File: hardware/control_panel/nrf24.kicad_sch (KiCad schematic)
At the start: 6 parts, among them J11 Conn_02x04_Odd_Even, U10 SPX3819M5-L-3-3

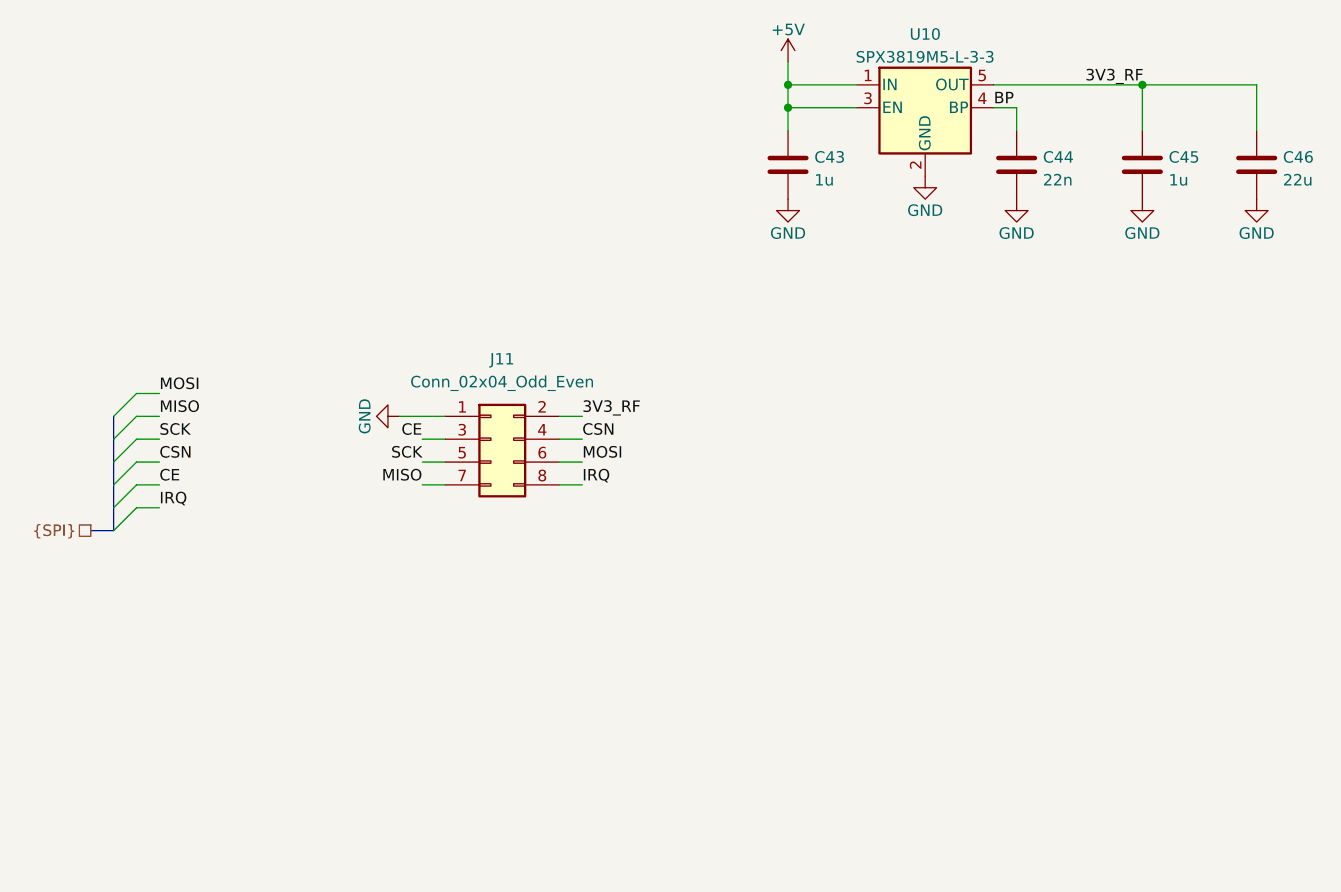
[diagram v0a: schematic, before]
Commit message: hw layout
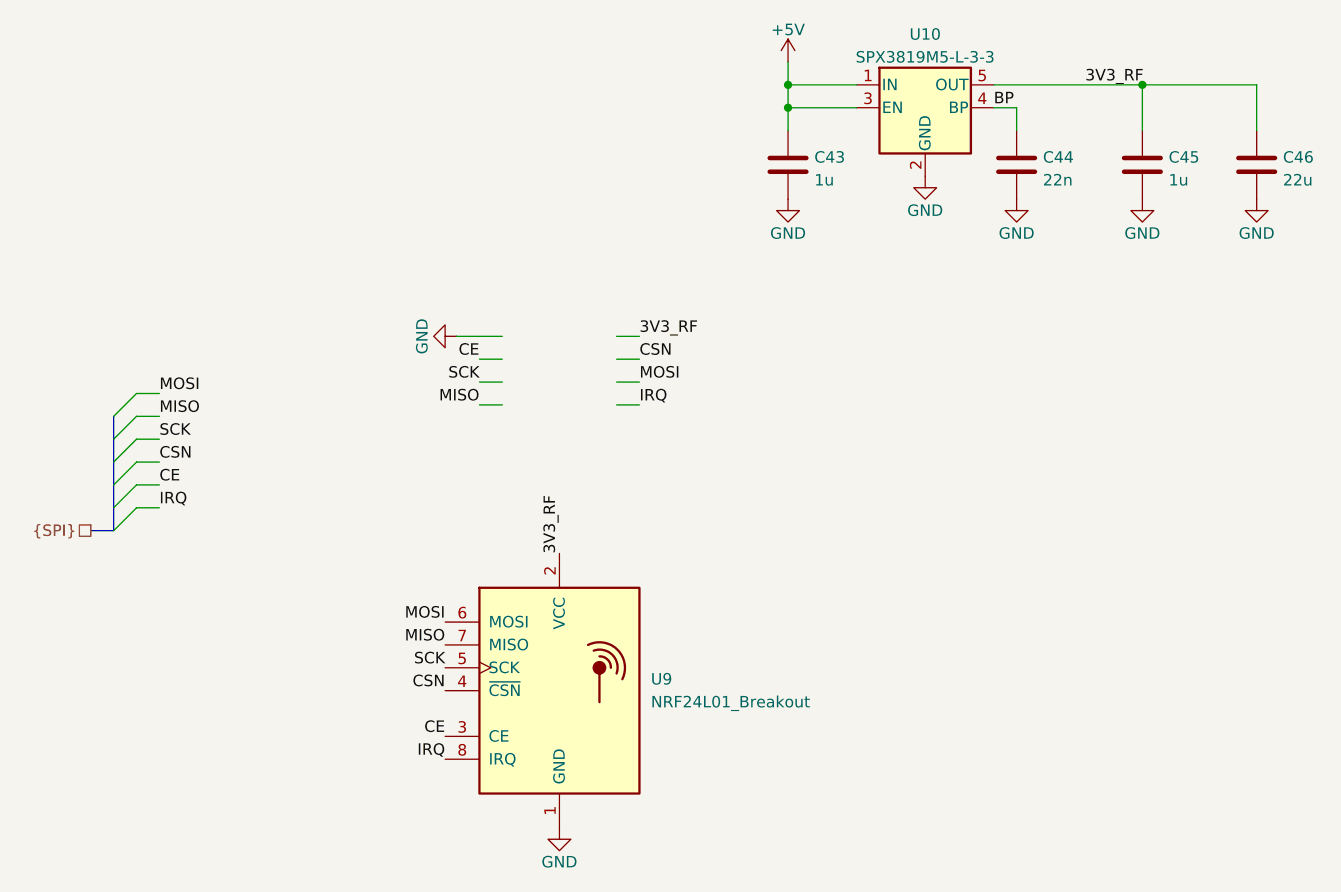
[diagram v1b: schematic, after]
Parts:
- removed J11: Conn_02x04_Odd_Even, Connector_PinSocket_2.54mm:PinSocket_2x04_P2.54mm_Vertical, symbol Connector_Generic:Conn_02x04_Odd_Even
- added U9: NRF24L01_Breakout, project_footprints:nRF24L01_Breakout, symbol RF:NRF24L01_Breakout
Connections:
- net 3V3_RF: now also U9.2 (VCC)
- net CE: now also U9.3 (CE)
- net CSN: now also U9.4 (~{CSN})
- net GND: now also U9.1 (GND)
- net IRQ: now also U9.8 (IRQ)
- net MISO: now also U9.7 (MISO)
- net MOSI: now also U9.6 (MOSI)
- net SCK: now also U9.5 (SCK)
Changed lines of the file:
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@@
     (stroke (width 0) (type default))
   )
-  (wire (pts (xy 113.03 81.28) (xy 110.49 81.28))
-    (stroke (width 0) (type default))
-  )
-  (wire (pts (xy 113.03 83.82) (xy 110.49 83.82))
-    (stroke (width 0) (type default))
-  )
-  (wire (pts (xy 95.25 81.28) (xy 97.79 81.28))
+  (wire (pts (xy 119.38 72.39) (xy 116.84 72.39))
+    (stroke (width 0) (type default))
+  )
+  (wire (pts (xy 119.38 74.93) (xy 116.84 74.93))
+    (stroke (width 0) (type default))
+  )
+  (wire (pts (xy 101.6 72.39) (xy 104.14 72.39))
     (stroke (width 0) (type default))
   )
@@
     (stroke (width 0) (type default))
   )
-  (wire (pts (xy 113.03 76.2) (xy 110.49 76.2))
+  (wire (pts (xy 119.38 67.31) (xy 116.84 67.31))
     (stroke (width 0) (type default))
   )
@@
     (stroke (width 0) (type default))
   )
-  (wire (pts (xy 113.03 78.74) (xy 110.49 78.74))
+  (wire (pts (xy 119.38 69.85) (xy 116.84 69.85))
     (stroke (width 0) (type default))
   )
@@
     (stroke (width 0) (type default))
   )
-  (wire (pts (xy 92.71 76.2) (xy 97.79 76.2))
-    (stroke (width 0) (type default))
-  )
-  (wire (pts (xy 95.25 78.74) (xy 97.79 78.74))
+  (wire (pts (xy 99.06 67.31) (xy 104.14 67.31))
+    (stroke (width 0) (type default))
+  )
+  (wire (pts (xy 101.6 69.85) (xy 104.14 69.85))
     (stroke (width 0) (type default))
   )
@@
     (stroke (width 0) (type default))
   )
-  (wire (pts (xy 95.25 83.82) (xy 97.79 83.82))
+  (wire (pts (xy 101.6 74.93) (xy 104.14 74.93))
     (stroke (width 0) (type default))
   )
@@
     (stroke (width 0) (type default))
   )
-  (label "MISO" (at 95.25 83.82 180) (fields_autoplaced)
+  (label "MISO" (at 101.6 74.93 180) (fields_autoplaced)
     (effects (font (size 1.27 1.27)) (justify right bottom))
   )
@@
     (effects (font (size 1.27 1.27)) (justify left bottom))
   )
-  (label "CSN" (at 113.03 78.74 0) (fields_autoplaced)
-    (effects (font (size 1.27 1.27)) (justify left bottom))
+  (label "IRQ" (at 97.79 114.3 180) (fields_autoplaced)
+    (effects (font (size 1.27 1.27)) (justify right bottom))
+  )
+  (label "CSN" (at 119.38 69.85 0) (fields_autoplaced)
+    (effects (font (size 1.27 1.27)) (justify left bottom))
+  )
+  (label "CSN" (at 97.79 106.68 180) (fields_autoplaced)
+    (effects (font (size 1.27 1.27)) (justify right bottom))
   )
   (label "CE" (at 66.04 83.82 0) (fields_autoplaced)
@@
     (effects (font (size 1.27 1.27)) (justify left bottom))
   )
-  (label "SCK" (at 95.25 81.28 180) (fields_autoplaced)
+  (label "SCK" (at 101.6 72.39 180) (fields_autoplaced)
     (effects (font (size 1.27 1.27)) (justify right bottom))
   )
@@
     (effects (font (size 1.27 1.27)) (justify left bottom))
   )
-  (label "3V3_RF" (at 113.03 76.2 0) (fields_autoplaced)
+  (label "MISO" (at 97.79 101.6 180) (fields_autoplaced)
+    (effects (font (size 1.27 1.27)) (justify right bottom))
+  )
+  (label "CE" (at 97.79 111.76 180) (fields_autoplaced)
+    (effects (font (size 1.27 1.27)) (justify right bottom))
+  )
+  (label "3V3_RF" (at 119.38 67.31 0) (fields_autoplaced)
     (effects (font (size 1.27 1.27)) (justify left bottom))
   )
@@
     (effects (font (size 1.27 1.27)) (justify left bottom))
   )
-  (label "IRQ" (at 113.03 83.82 0) (fields_autoplaced)
+  (label "IRQ" (at 119.38 74.93 0) (fields_autoplaced)
     (effects (font (size 1.27 1.27)) (justify left bottom))
   )
@@
     (effects (font (size 1.27 1.27)) (justify left bottom))
   )
-  (label "CE" (at 95.25 78.74 180) (fields_autoplaced)
+  (label "3V3_RF" (at 110.49 91.44 90) (fields_autoplaced)
+    (effects (font (size 1.27 1.27)) (justify left bottom))
+  )
+  (label "CE" (at 101.6 69.85 180) (fields_autoplaced)
     (effects (font (size 1.27 1.27)) (justify right bottom))
   )
@@
     (effects (font (size 1.27 1.27)) (justify left bottom))
   )
-  (label "MOSI" (at 113.03 81.28 0) (fields_autoplaced)
+  (label "MOSI" (at 97.79 99.06 180) (fields_autoplaced)
+    (effects (font (size 1.27 1.27)) (justify right bottom))
+  )
+  (label "MOSI" (at 119.38 72.39 0) (fields_autoplaced)
     (effects (font (size 1.27 1.27)) (justify left bottom))
   )
   (label "IRQ" (at 66.04 86.36 0) (fields_autoplaced)
     (effects (font (size 1.27 1.27)) (justify left bottom))
+  )
+  (label "SCK" (at 97.79 104.14 180) (fields_autoplaced)
+    (effects (font (size 1.27 1.27)) (justify right bottom))
   )
   (hierarchical_label "{SPI}" (shape passive) (at 58.42 88.9 180) (fields_autoplaced)
@@
     )
   )
-  (symbol (lib_id "power:GND") (at 92.71 76.2 270) (mirror x) (unit 1)
+  (symbol (lib_id "power:GND") (at 99.06 67.31 270) (mirror x) (unit 1)
     (in_bom yes) (on_board yes) (dnp no)
-    (property "Reference" "#PWR0195" (at 86.36 76.2 0)
-      (effects (font (size 1.27 1.27)) hide)
-    )
-    (property "Value" "GND" (at 88.9 76.2 0)
-      (effects (font (size 1.27 1.27)))
-    )
-    (property "Footprint" "" (at 92.71 76.2 0)
-      (effects (font (size 1.27 1.27)) hide)
-    )
-    (property "Datasheet" "" (at 92.71 76.2 0)
+    (property "Reference" "#PWR0195" (at 92.71 67.31 0)
+      (effects (font (size 1.27 1.27)) hide)
+    )
+    (property "Value" "GND" (at 95.25 67.31 0)
+      (effects (font (size 1.27 1.27)))
+    )
+    (property "Footprint" "" (at 99.06 67.31 0)
+      (effects (font (size 1.27 1.27)) hide)
+    )
+    (property "Datasheet" "" (at 99.06 67.31 0)
       (effects (font (size 1.27 1.27)) hide)
     )
@@
     )
   )
-  (symbol (lib_id "Connector_Generic:Conn_02x04_Odd_Even") (at 102.87 78.74 0) (unit 1)
+  (symbol (lib_id "Regulator_Linear:SPX3819M5-L-3-3") (at 151.13 41.91 0) (unit 1)
     (in_bom yes) (on_board yes) (dnp no) (fields_autoplaced)
-    (property "Reference" "J11" (at 104.14 69.85 0)
-      (effects (font (size 1.27 1.27)))
-    )
-    (property "Value" "Conn_02x04_Odd_Even" (at 104.14 72.39 0)
-      (effects (font (size 1.27 1.27)))
-    )
-    (property "Footprint" "Connector_PinSocket_2.54mm:PinSocket_2x04_P2.54mm_Vertical" (at 102.87 78.74 0)
-      (effects (font (size 1.27 1.27)) hide)
-    )
-    (property "Datasheet" "~" (at 102.87 78.74 0)
+    (property "Reference" "U10" (at 151.13 33.7652 0)
+      (effects (font (size 1.27 1.27)))
+    )
+    (property "Value" "SPX3819M5-L-3-3" (at 151.13 36.3021 0)
+      (effects (font (size 1.27 1.27)))
+    )
+    (property "Footprint" "Package_TO_SOT_SMD:SOT-23-5" (at 151.13 33.655 0)
+      (effects (font (size 1.27 1.27)) hide)
+    )
+    (property "Datasheet" "https://www.exar.com/content/document.ashx?id=22106&languageid=1033&type=Datasheet&partnumber=SPX3819&filename=SPX3819.pdf&part=SPX3819" (at 151.13 41.91 0)
+      (effects (font (size 1.27 1.27)) hide)
+    )
+    (pin "1")
+    (pin "2")
+    (pin "3")
+    (pin "4")
+    (pin "5")
+    (instances
+      (project "control_panel"
+        (path "/e63e39d7-6ac0-4ffd-8aa3-1841a4541b55/6e17d1e8-6187-4b57-9ae7-c92547e687f9"
+          (reference "U10") (unit 1)
+        )
+      )
+    )
+  )
+  (symbol (lib_id "RF:NRF24L01_Breakout") (at 110.49 106.68 0) (unit 1)
+    (in_bom yes) (on_board yes) (dnp no) (fields_autoplaced)
+    (property "Reference" "U9" (at 120.65 105.41 0)
+      (effects (font (size 1.27 1.27)) (justify left))
+    )
+    (property "Value" "NRF24L01_Breakout" (at 120.65 107.95 0)
+      (effects (font (size 1.27 1.27)) (justify left))
+    )
+    (property "Footprint" "project_footprints:nRF24L01_Breakout" (at 114.3 91.44 0)
+      (effects (font (size 1.27 1.27) italic) (justify left) hide)
+    )
+    (property "Datasheet" "http://www.nordicsemi.com/eng/content/download/2730/34105/file/nRF24L01_Product_Specification_v2_0.pdf" (at 110.49 109.22 0)
       (effects (font (size 1.27 1.27)) hide)
     )
@@
       (project "control_panel"
         (path "/e63e39d7-6ac0-4ffd-8aa3-1841a4541b55/6e17d1e8-6187-4b57-9ae7-c92547e687f9"
-          (reference "J11") (unit 1)
-        )
-      )
-    )
-  )
-  (symbol (lib_id "Regulator_Linear:SPX3819M5-L-3-3") (at 151.13 41.91 0) (unit 1)
-    (in_bom yes) (on_board yes) (dnp no) (fields_autoplaced)
-    (property "Reference" "U10" (at 151.13 33.7652 0)
-      (effects (font (size 1.27 1.27)))
-    )
-    (property "Value" "SPX3819M5-L-3-3" (at 151.13 36.3021 0)
-      (effects (font (size 1.27 1.27)))
-    )
-    (property "Footprint" "Package_TO_SOT_SMD:SOT-23-5" (at 151.13 33.655 0)
-      (effects (font (size 1.27 1.27)) hide)
-    )
-    (property "Datasheet" "https://www.exar.com/content/document.ashx?id=22106&languageid=1033&type=Datasheet&partnumber=SPX3819&filename=SPX3819.pdf&part=SPX3819" (at 151.13 41.91 0)
-      (effects (font (size 1.27 1.27)) hide)
-    )
-    (pin "1")
-    (pin "2")
-    (pin "3")
-    (pin "4")
-    (pin "5")
-    (instances
-      (project "control_panel"
-        (path "/e63e39d7-6ac0-4ffd-8aa3-1841a4541b55/6e17d1e8-6187-4b57-9ae7-c92547e687f9"
-          (reference "U10") (unit 1)
+          (reference "U9") (unit 1)
         )
       )
@@
         )
       )
+    )
+  )
+  (symbol (lib_id "power:GND") (at 110.49 121.92 0) (mirror y) (unit 1)
+    (in_bom yes) (on_board yes) (dnp no)
+    (property "Reference" "#PWR047" (at 110.49 128.27 0)
+      (effects (font (size 1.27 1.27)) hide)
+    )
+    (property "Value" "GND" (at 110.49 125.73 0)
+      (effects (font (size 1.27 1.27)))
+    )
+    (property "Footprint" "" (at 110.49 121.92 0)
+      (effects (font (size 1.27 1.27)) hide)
+    )
+    (property "Datasheet" "" (at 110.49 121.92 0)
+      (effects (font (size 1.27 1.27)) hide)
+    )
+    (pin "1")
+    (instances
+      (project "control_panel"
+        (path "/e63e39d7-6ac0-4ffd-8aa3-1841a4541b55/6e17d1e8-6187-4b57-9ae7-c92547e687f9"
+          (reference "#PWR047") (unit 1)
+        )
+      )
